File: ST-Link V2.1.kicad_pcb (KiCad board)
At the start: 2 copper layers, 33.6 x 21.1 mm, 45 parts, among them J1 USB_OTG, J2 Conn_01x06, J3 Conn_01x08, J4 Conn_01x08, Q1 MMBT3904, U1 USBLC6-2SC6, U2 stm32, U3 MIC5219-3.3, X1 8MHz

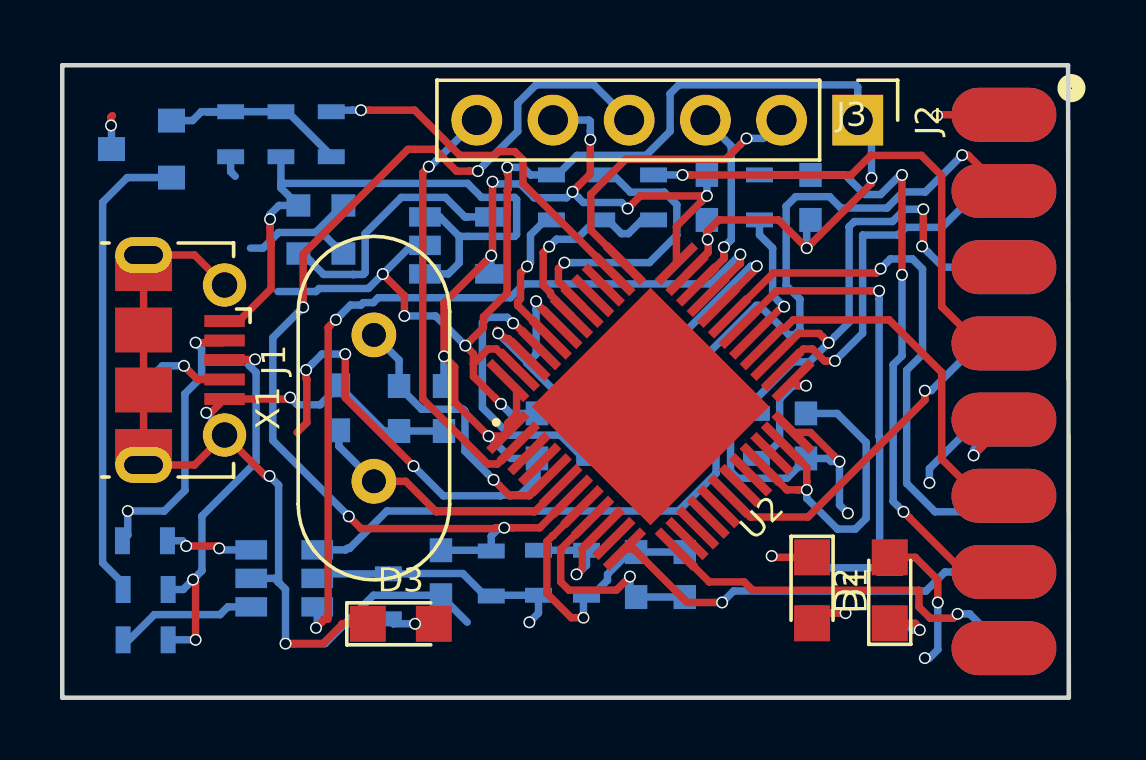
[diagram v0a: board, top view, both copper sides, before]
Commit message: save for reroute
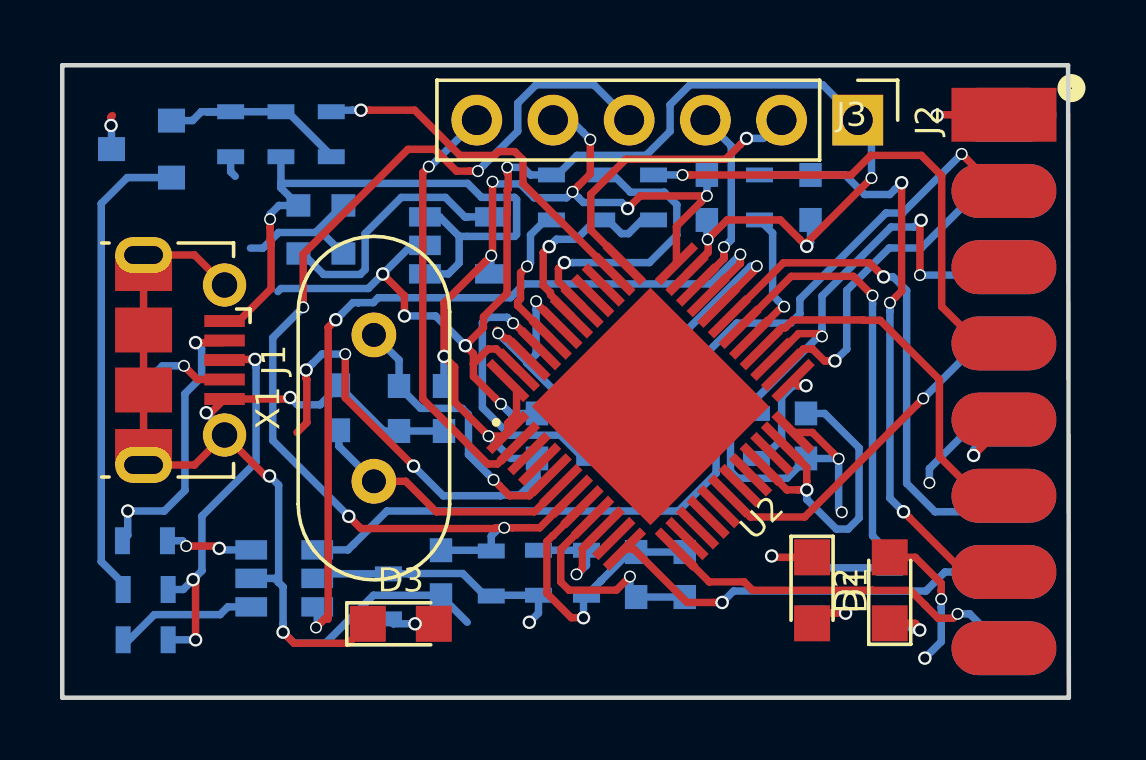
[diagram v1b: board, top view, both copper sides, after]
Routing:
- net /T_SWIM: track 20.3 -> 16.4 mm
- net GND: track 124.5 -> 122.7 mm
- net /T_SWO: track 19.6 -> 18.3 mm
- net /T_SWDIO_JTMS: track 17.2 -> 16.1 mm
- net /T_SWCLK_JTCK: track 12.1 -> 11.3 mm
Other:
- net class Default: via_dia 0.4 -> 0.45

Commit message: route route route
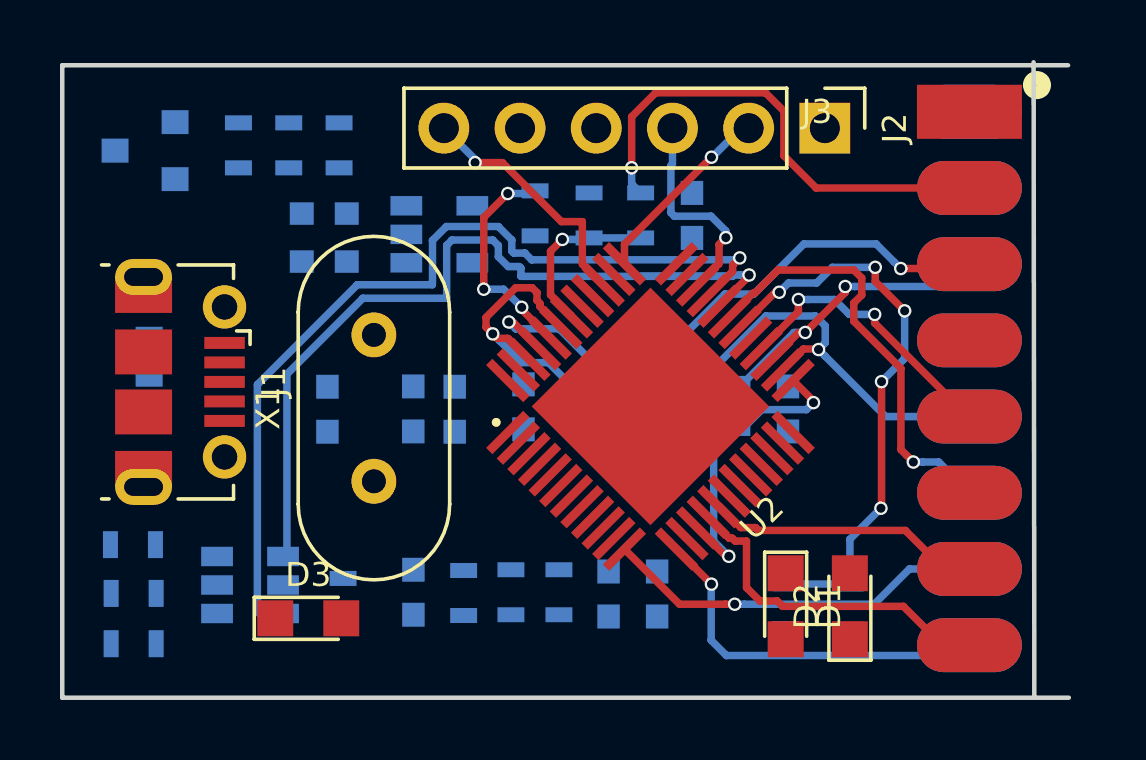
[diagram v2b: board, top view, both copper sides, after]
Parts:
- removed C7: 20pF, Capacitors_SMD:C_0603
- removed R15: 20, Resistors_SMD:R_0603
- moved D3 3.09 mm to (126.3, 116.5)
- moved R16 1.52 mm to (127.5, 115.9)
- moved D2 1.43 mm to (144.4, 116.1)
- moved R13 1.43 mm to (144.4, 116.1)
- moved R14 1.19 mm to (140.6, 109.4)
- moved U1 1.16 mm to (124.4, 115.4)
- moved J3 1.15 mm to (148.3, 99.6)
- moved J4 1.15 mm to (148.3, 99.6)
- moved J2 1.13 mm to (143.5, 100.1)
- moved C12 1.13 mm to (137.9, 115.7)
- moved C8 1.13 mm to (136.3, 115.7)
- moved R1 1.13 mm to (131.5, 115.6)
- moved C1 1.13 mm to (129.8, 115.6)
- moved R3 1.13 mm to (133.1, 115.6)
- moved R2 1.13 mm to (134.7, 115.6)
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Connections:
- J2 pad 6: /PC13 -> /STM_SWO
- J3 pad 2: /T_SWIM -> /T_RESET
- J3 pad 3: Net-(J3-Pad3) -> /T_SWIM
- J3 pad 4: /T_RESET -> /3V3_ST_LINK
- J3 pad 5: /3V3_ST_LINK -> /PWR_ENn
- J3 pad 6: /PWR_ENn -> /T_JRST
- J3 pad 7: /MCO -> /T_JTDI
- J3 pad 8: Net-(J3-Pad8) -> /T_JTDO
- J4 pad 2: /T_SWCLK_JTCK -> /T_NRST
- J4 pad 4: /T_NRST -> /3V3_ST_LINK
- J4 pad 5: /3V3_ST_LINK -> /T_SWCLK_JTCK
- U2 pad 15: Net-(U2-Pad15) -> /T_SWCLK_JTCK
- U2 pad 16: Net-(U2-Pad16) -> /T_JTDO
- U2 pad 17: Net-(U2-Pad17) -> /T_JTDI
- U2 pad 19: Net-(U2-Pad19) -> /T_JRST
- U2 pad 2: /PC13 -> Net-(U2-Pad2)
- U2 pad 39: Net-(U2-Pad39) -> /STM_SWO
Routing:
- net GND: track 122.7 -> 0.00 mm, vias 16 -> 0
- net /3V3_ST_LINK: track 84.4 -> 0.00 mm, vias 20 -> 0
- net /NRST: track 36.4 -> 0.00 mm, vias 4 -> 0
- net +5V: track 22.3 -> 0.00 mm, vias 1 -> 0
- net /MCO: track 21.7 -> 0.00 mm, vias 3 -> 0
- net Net-(Q1-Pad2): track 15.9 -> 0.00 mm
- net /PC13: track 14.4 -> 0.00 mm, vias 1 -> 0
- net Net-(J1-Pad3): track 13.2 -> 0.00 mm, vias 3 -> 0
- net /USB_RENUMN: track 12.3 -> 0.00 mm, vias 1 -> 0
- net /T_NRST: track 11.8 -> 0.00 mm, vias 1 -> 0
- net /T_JTDO: track 0.00 -> 11.4 mm
- net /SWIM_RST_IN: track 10.1 -> 0.00 mm, vias 1 -> 0
- net Net-(C3-Pad2): track 9.69 -> 0.00 mm, vias 1 -> 0
- net /T_SWCLK_JTCK: track 11.3 -> 20.8 mm, vias 1 -> 2
- net Net-(J1-Pad2): track 9.49 -> 0.00 mm, vias 2 -> 0
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- removed copper zone on F.Cu, net /3V3_ST_LINK
- removed copper zone on B.Cu, net GND
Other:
- board size 33.6 x 21.1 mm -> 33.6 x 21.2 mm
